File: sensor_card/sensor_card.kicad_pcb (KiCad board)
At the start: 2 copper layers, 56 x 86 mm, 10 parts, among them J1 Raspberry_Pi_4, J10 Conn_01x05, J2 BME280, J3 GPS, J4 PARACHUTE, J5 Conn_01x02, J6 power LORA, J7 power_RPI, J8 MPU_6500, U1 Ai-Thinker-Ra-02

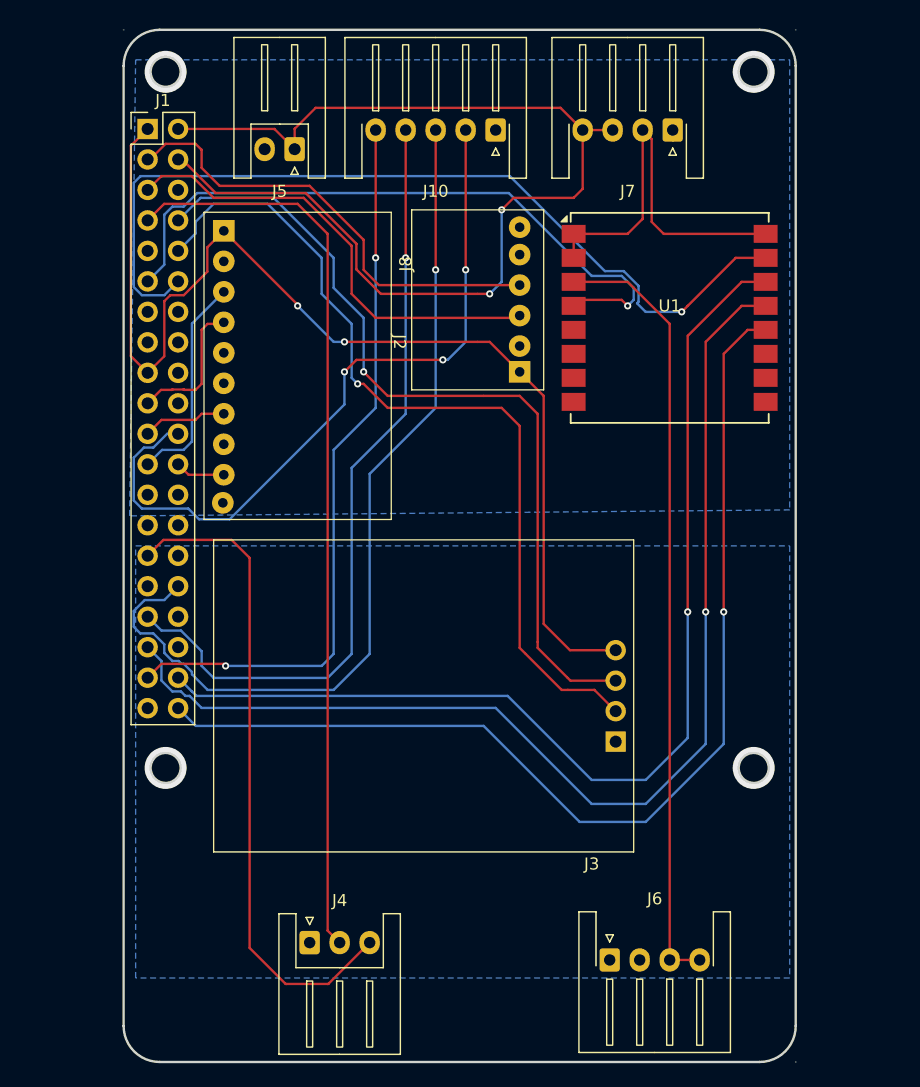
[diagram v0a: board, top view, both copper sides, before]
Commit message: Fully Routed Sensor board
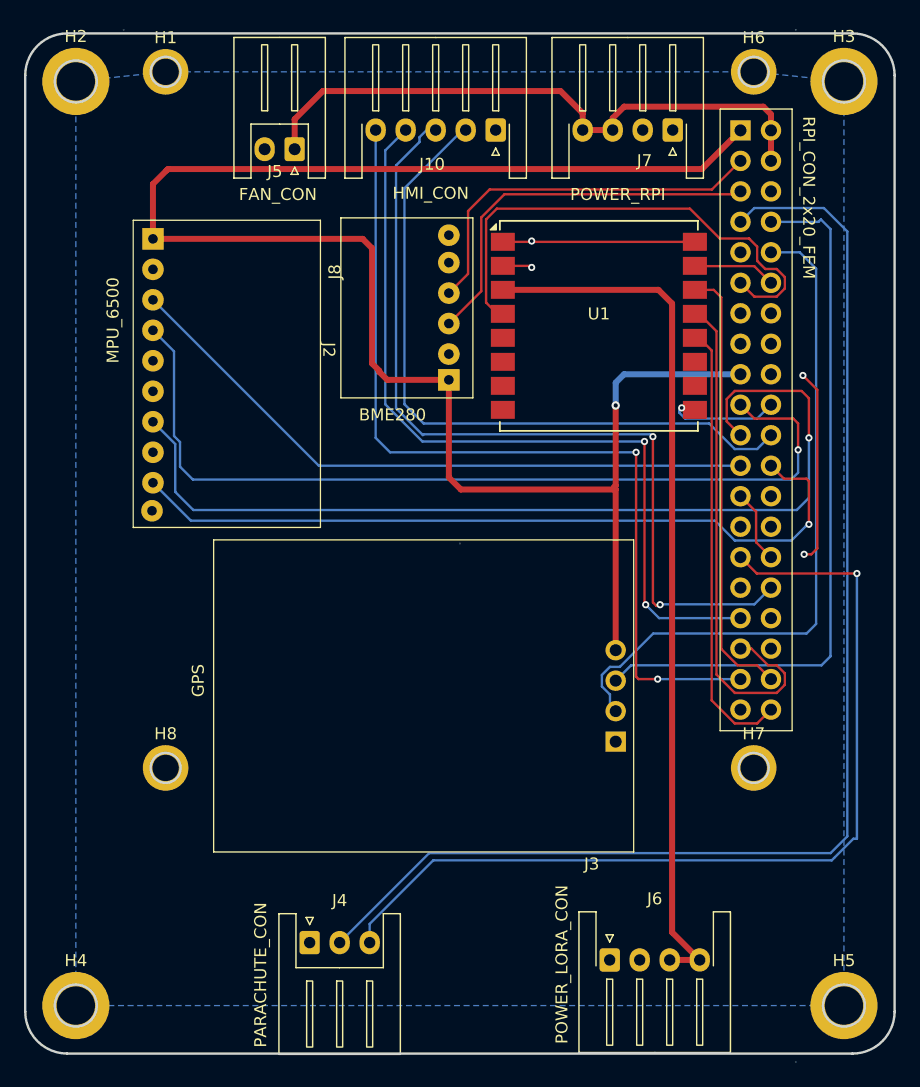
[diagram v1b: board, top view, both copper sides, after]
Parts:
- added H1: MountingHole_RPI, MountingHole:MountingHole_2.2mm_M2_DIN965_Pad, F.Cu at (82.5, 41.5)
- added H2: MountingHole_Pad, MountingHole:MountingHole_3.2mm_M3_DIN965_Pad, F.Cu at (75.0, 42.3)
- added H3: MountingHole_Pad, MountingHole:MountingHole_3.2mm_M3_DIN965_Pad, F.Cu at (139.0, 42.3)
- added H4: MountingHole_Pad, MountingHole:MountingHole_3.2mm_M3_DIN965_Pad, F.Cu at (75.0, 119.3)
- added H5: MountingHole_Pad, MountingHole:MountingHole_3.2mm_M3_DIN965_Pad, F.Cu at (139.0, 119.3)
- added H6: MountingHole_RPI, MountingHole:MountingHole_2.2mm_M2_DIN965_Pad, F.Cu at (131.5, 41.5)
- added H7: MountingHole_RPI, MountingHole:MountingHole_2.2mm_M2_DIN965_Pad, F.Cu at (131.5, 99.5)
- added H8: MountingHole_RPI, MountingHole:MountingHole_2.2mm_M2_DIN965_Pad, F.Cu at (82.5, 99.5)
- J1: footprint Connector_PinHeader_2.54mm:PinHeader_2x20_P2.54mm_Vertical -> Connector_PinSocket_2.54mm:PinSocket_2x20_P2.54mm_Vertical; moved to B.Cu
- moved J1 49.4 mm to (130.4, 46.4), turned to 180 degrees
- moved J2 5.94 mm to (102.1, 58.7)
- moved J8 5.94 mm to (87.6, 66.2)
- moved U1 5.94 mm to (118.6, 62.7)
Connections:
- J1 pad 15: /LED_ALIM_PARA -> unconnected-(J1-GPIO22/SDIO_CLK-Pad15)
- J1 pad 16: /LED_OUVERT_PARA -> unconnected-(J1-GPIO23/SDIO_CMD-Pad16)
- J1 pad 18: /LED_DECL_PARA -> unconnected-(J1-GPIO24/SDIO_DAT0-Pad18)
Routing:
- net /MPU_MISO: track 7.04 -> 79.7 mm, vias 0 -> 1
- net /LORA_CS: track 73.6 -> 6.93 mm, vias 1 -> 0
- net /MPU_MOSI: track 11.8 -> 74.0 mm, vias 0 -> 1
- net /MPU_CS: track 4.17 -> 64.5 mm, vias 0 -> 1
- net /LORA_MOSI: track 89.3 -> 36.9 mm, vias 1 -> 0
- net /LORA_SCK: track 88.9 -> 37.2 mm, vias 1 -> 0
- net /LORA_MISO: track 94.7 -> 43.1 mm, vias 1 -> 0
- net +3V3: track 94.9 -> 146.1 mm, vias 2 -> 1
- net +5V: track 91.7 -> 50.9 mm, vias 2 -> 0
- net /MPU_SCK: track 18.1 -> 54.7 mm
- net /PARACHUTE_ACTIVATION: track 76.1 -> 106.6 mm
- net /PARA_STATE_FEEDBACK: track 54.8 -> 77.5 mm, vias 0 -> 1
- net GND: track 34.4 -> 50.8 mm, vias 0 -> 5
- net /GPS_TX: track 71.4 -> 57.0 mm, vias 1 -> 0
- net /LED_FONC_PROGRAMMES: track 61.6 -> 75.3 mm
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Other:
- board size 56 x 86 mm -> 72.4 x 86 mm
- board text added: "BME280"
- board text added: "FAN_CON"
- board text added: "GPS"
- board text added: "HMI_CON"
- board text added: "LORA"
- board text added: "MPU_6500"
- board text added: "PARACHUTE_CON"
- board text added: "POWER_LORA_CON"
- board text added: "POWER_RPI"
- board text added: "RPI_CON_2x20_FEM"
